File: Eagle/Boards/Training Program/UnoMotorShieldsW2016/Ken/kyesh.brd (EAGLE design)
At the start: 100 x 80 mm, 5 parts, among them J1 ARDUINO_UNO_R3

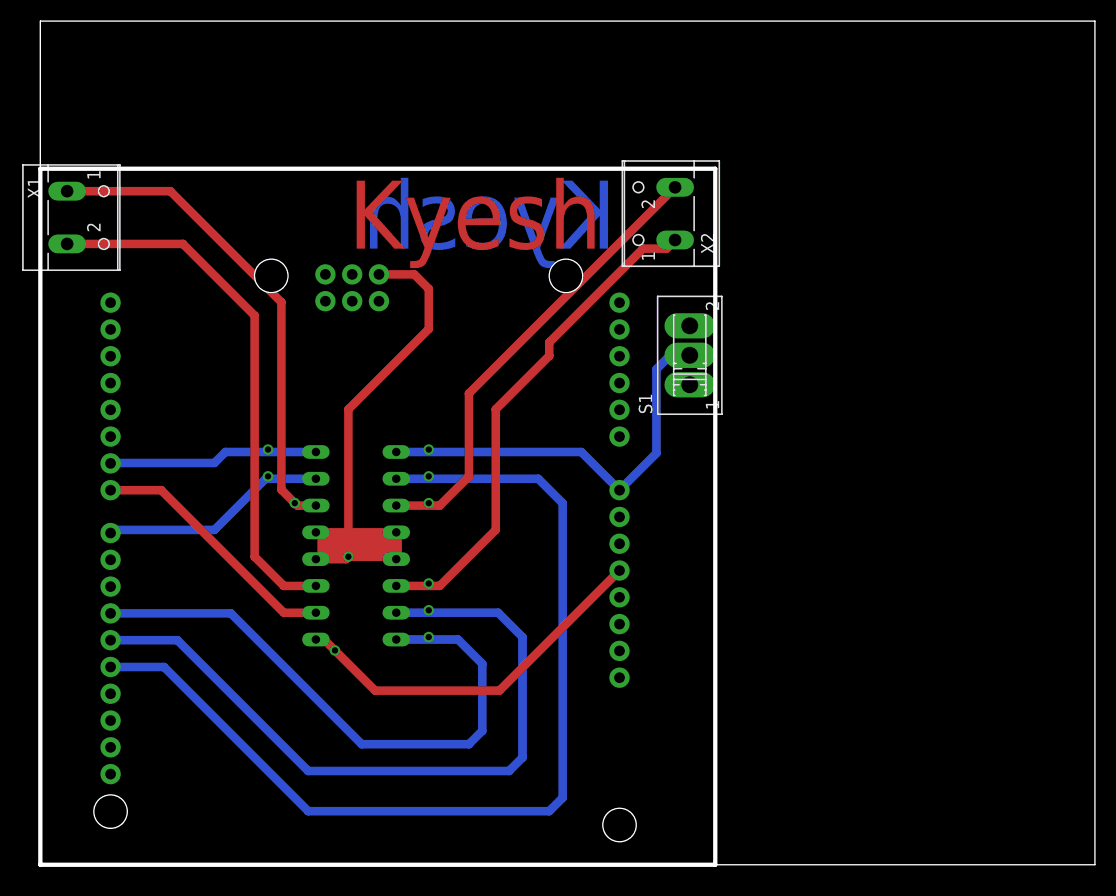
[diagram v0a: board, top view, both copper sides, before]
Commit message: compiled 1st board for fabrication
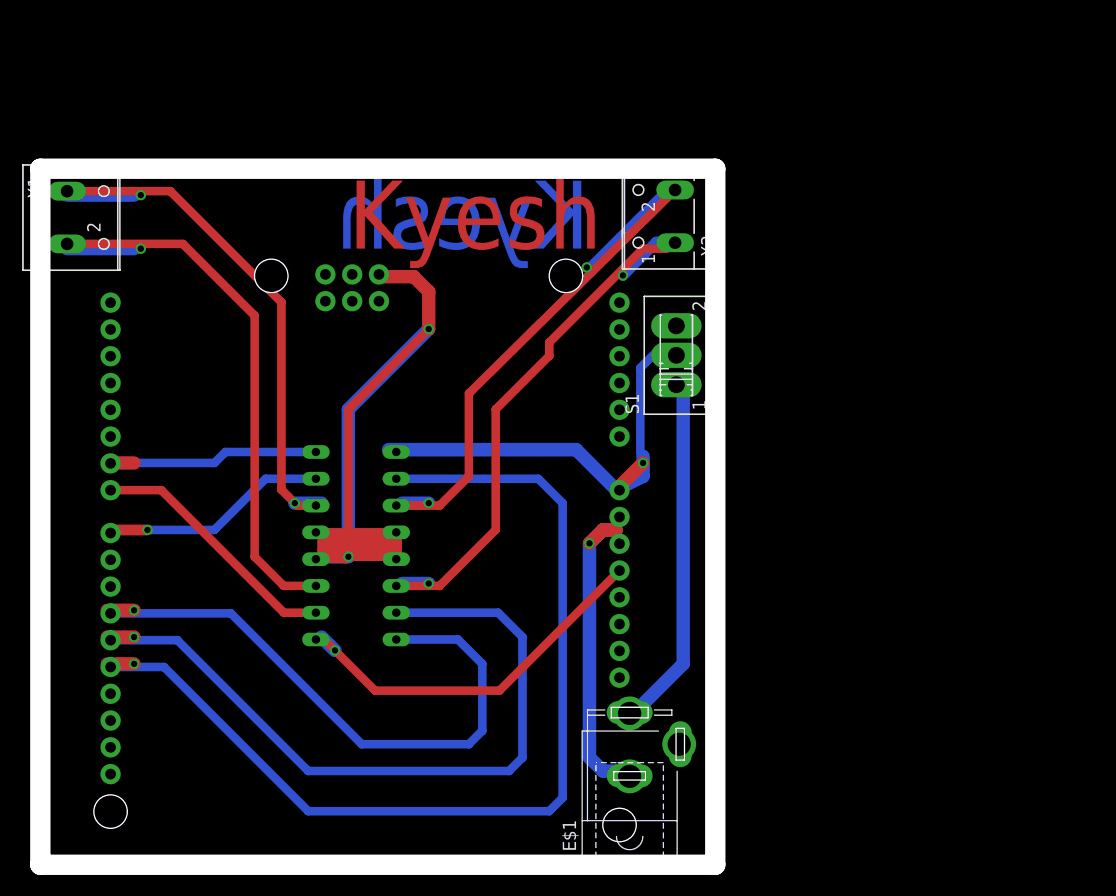
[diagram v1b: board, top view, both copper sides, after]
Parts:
- added E$1: (no value), ISCTRainingProgram:5.5-2.5-BARRELCONNECTOR
- moved S1 1.27 mm to (60.3, 48.3)
- moved X2 0.25 mm to (58.9, 61.5)
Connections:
- new net S$15: S1.2
- net N$4: no longer S1.2
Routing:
- net N$2: track 37.0 -> 73.3 mm, vias 1 -> 2
- net S$1: track 0.00 -> 33.9 mm
- net S$2: track 0.00 -> 30.8 mm, vias 0 -> 1
- net N$4: track 39.3 -> 58.2 mm, vias 0 -> 1
- net S$13: track 0.00 -> 10.8 mm
- net S$14: track 0.00 -> 10.3 mm
- net S$12: track 0.00 -> 6.35 mm
- net S$11: track 0.00 -> 6.35 mm
- net S$8: track 0.00 -> 5.13 mm, vias 0 -> 1
- net N$8: track 21.6 -> 25.4 mm, vias 0 -> 1
- net S$6: track 0.00 -> 2.54 mm, vias 0 -> 1
- net S$5: track 0.00 -> 2.54 mm, vias 0 -> 1
- net S$4: track 0.00 -> 2.54 mm, vias 0 -> 1
- net S$3: track 0.00 -> 2.54 mm
- net N$6: track 46.4 -> 48.9 mm
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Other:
- board size 100 x 80 mm -> 64 x 66 mm
